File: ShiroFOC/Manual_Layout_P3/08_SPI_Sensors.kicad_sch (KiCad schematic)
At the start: 15 parts, among them U601 AS5047P-ATSM, U701 BMI323

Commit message: CAN layout
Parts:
- C601: symbol Manual:COMP_C601 -> ShiroFOCLib:COMP_C601
- C602: symbol Manual:COMP_C602 -> ShiroFOCLib:COMP_C602
- C701: symbol Manual:COMP_C701 -> ShiroFOCLib:COMP_C701
- C702: symbol Manual:COMP_C702 -> ShiroFOCLib:COMP_C702
- R308, R715: symbol Manual:COMP_R308 -> ShiroFOCLib:COMP_R308
- R309: symbol Manual:COMP_R309 -> ShiroFOCLib:COMP_R309
- R313: symbol Manual:COMP_R313 -> ShiroFOCLib:COMP_R313
- R314: symbol Manual:COMP_R314 -> ShiroFOCLib:COMP_R314
- R611: symbol Manual:COMP_R611 -> ShiroFOCLib:COMP_R611
- TP1010: symbol Manual:COMP_TP1010 -> ShiroFOCLib:COMP_TP1010
- TP1011: symbol Manual:COMP_TP1011 -> ShiroFOCLib:COMP_TP1011
- TP1012: symbol Manual:COMP_TP1012 -> ShiroFOCLib:COMP_TP1012
- U601: footprint Manual:AS5047P_TSSOP14 -> ShiroFOCLib:AS5047P_TSSOP14; symbol Manual:COMP_U601 -> ShiroFOCLib:COMP_U601
- U701: footprint Manual:BMI323_LGA14 -> ShiroFOCLib:BMI323_LGA14; symbol Manual:COMP_U701_I2C -> ShiroFOCLib:COMP_U701_I2C
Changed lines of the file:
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@@
 	)
 	(symbol
-		(lib_id "Manual:COMP_C702")
+		(lib_id "ShiroFOCLib:COMP_C702")
 		(at 195.58 168.91 0)
 		(unit 1)
@@
 	)
 	(symbol
-		(lib_id "Manual:COMP_TP1012")
+		(lib_id "ShiroFOCLib:COMP_TP1012")
 		(at 120.65 93.98 0)
 		(unit 1)
@@
 	)
 	(symbol
-		(lib_id "Manual:COMP_TP1011")
+		(lib_id "ShiroFOCLib:COMP_TP1011")
 		(at 109.22 104.14 0)
 		(unit 1)
@@
 	)
 	(symbol
-		(lib_id "Manual:PWR_3V3")
+		(lib_id "ShiroFOCLib:PWR_3V3")
 		(at 154.94 38.1 0)
 		(unit 1)
@@
 	)
 	(symbol
-		(lib_id "Manual:PWR_3V3")
+		(lib_id "ShiroFOCLib:PWR_3V3")
 		(at 180.34 180.34 0)
 		(unit 1)
@@
 	)
 	(symbol
-		(lib_id "Manual:PWR_3V3")
+		(lib_id "ShiroFOCLib:PWR_3V3")
 		(at 96.52 177.8 0)
 		(unit 1)
@@
 	)
 	(symbol
-		(lib_id "Manual:PWR_GND")
+		(lib_id "ShiroFOCLib:PWR_GND")
 		(at 180.34 137.16 0)
 		(unit 1)
@@
 	)
 	(symbol
-		(lib_id "Manual:COMP_U601")
+		(lib_id "ShiroFOCLib:COMP_U601")
 		(at 175.26 96.52 0)
 		(unit 1)
@@
 			)
 		)
-		(property "Footprint" "Manual:AS5047P_TSSOP14"
+		(property "Footprint" "ShiroFOCLib:AS5047P_TSSOP14"
 			(at 175.26 129.54 0)
 			(effects
@@
 	)
 	(symbol
-		(lib_id "Manual:COMP_R309")
+		(lib_id "ShiroFOCLib:COMP_R309")
 		(at 223.52 59.69 0)
 		(unit 1)
@@
 	)
 	(symbol
-		(lib_id "Manual:PWR_GND")
+		(lib_id "ShiroFOCLib:PWR_GND")
 		(at 170.18 246.38 0)
 		(unit 1)
@@
 	)
 	(symbol
-		(lib_id "Manual:COMP_R313")
+		(lib_id "ShiroFOCLib:COMP_R313")
 		(at 101.6 83.82 0)
 		(unit 1)
@@
 	)
 	(symbol
-		(lib_id "Manual:COMP_C601")
+		(lib_id "ShiroFOCLib:COMP_C601")
 		(at 154.94 48.26 0)
 		(unit 1)
@@
 	)
 	(symbol
-		(lib_id "Manual:PWR_3V3")
+		(lib_id "ShiroFOCLib:PWR_3V3")
 		(at 180.34 55.88 0)
 		(unit 1)
@@
 	)
 	(symbol
-		(lib_id "Manual:PWR_3V3")
+		(lib_id "ShiroFOCLib:PWR_3V3")
 		(at 170.18 55.88 0)
 		(unit 1)
@@
 	)
 	(symbol
-		(lib_id "Manual:COMP_C602")
+		(lib_id "ShiroFOCLib:COMP_C602")
 		(at 195.58 48.26 0)
 		(unit 1)
@@
 	)
 	(symbol
-		(lib_id "Manual:PWR_3V3")
+		(lib_id "ShiroFOCLib:PWR_3V3")
 		(at 223.52 187.96 0)
 		(unit 1)
@@
 	)
 	(symbol
-		(lib_id "Manual:PWR_GND")
+		(lib_id "ShiroFOCLib:PWR_GND")
 		(at 170.18 137.16 0)
 		(unit 1)
@@
 	)
 	(symbol
-		(lib_id "Manual:COMP_C701")
+		(lib_id "ShiroFOCLib:COMP_C701")
 		(at 154.94 168.91 0)
 		(unit 1)
@@
 	)
 	(symbol
-		(lib_id "Manual:COMP_R308")
+		(lib_id "ShiroFOCLib:COMP_R308")
 		(at 96.52 187.96 0)
 		(unit 1)
@@
 	)
 	(symbol
-		(lib_id "Manual:PWR_GND")
+		(lib_id "ShiroFOCLib:PWR_GND")
 		(at 148.59 226.06 0)
 		(unit 1)
@@
 	)
 	(symbol
-		(lib_id "Manual:PWR_GND")
+		(lib_id "ShiroFOCLib:PWR_GND")
 		(at 154.94 58.42 0)
 		(unit 1)
@@
 	)
 	(symbol
-		(lib_id "Manual:PWR_GND")
+		(lib_id "ShiroFOCLib:PWR_GND")
 		(at 195.58 179.07 0)
 		(unit 1)
@@
 	)
 	(symbol
-		(lib_id "Manual:COMP_R308")
+		(lib_id "ShiroFOCLib:COMP_R308")
 		(at 121.92 187.96 0)
 		(unit 1)
@@
 	)
 	(symbol
-		(lib_id "Manual:PWR_3V3")
+		(lib_id "ShiroFOCLib:PWR_3V3")
 		(at 195.58 38.1 0)
 		(unit 1)
@@
 	)
 	(symbol
-		(lib_id "Manual:COMP_R611")
+		(lib_id "ShiroFOCLib:COMP_R611")
 		(at 130.81 104.14 0)
 		(unit 1)
@@
 	)
 	(symbol
-		(lib_id "Manual:PWR_3V3")
+		(lib_id "ShiroFOCLib:PWR_3V3")
 		(at 121.92 177.8 0)
 		(unit 1)
@@
 	)
 	(symbol
-		(lib_id "Manual:PWR_GND")
+		(lib_id "ShiroFOCLib:PWR_GND")
 		(at 180.34 246.38 0)
 		(unit 1)
@@
 	)
 	(symbol
-		(lib_id "Manual:COMP_TP1010")
+		(lib_id "ShiroFOCLib:COMP_TP1010")
 		(at 120.65 83.82 0)
 		(unit 1)
@@
 	)
 	(symbol
-		(lib_id "Manual:PWR_GND")
+		(lib_id "ShiroFOCLib:PWR_GND")
 		(at 154.94 179.07 0)
 		(unit 1)
@@
 	)
 	(symbol
-		(lib_id "Manual:PWR_3V3")
+		(lib_id "ShiroFOCLib:PWR_3V3")
 		(at 223.52 49.53 0)
 		(unit 1)
@@
 	)
 	(symbol
-		(lib_id "Manual:PWR_3V3")
+		(lib_id "ShiroFOCLib:PWR_3V3")
 		(at 195.58 158.75 0)
 		(unit 1)
@@
 	)
 	(symbol
-		(lib_id "Manual:PWR_3V3")
+		(lib_id "ShiroFOCLib:PWR_3V3")
 		(at 170.18 180.34 0)
 		(unit 1)
@@
 	)
 	(symbol
-		(lib_id "Manual:COMP_U701_I2C")
+		(lib_id "ShiroFOCLib:COMP_U701_I2C")
 		(at 175.26 213.36 0)
 		(unit 1)
@@
 			)
 		)
-		(property "Footprint" "Manual:BMI323_LGA14"
+		(property "Footprint" "ShiroFOCLib:BMI323_LGA14"
 			(at 175.26 238.76 0)
 			(effects
@@
 	)
 	(symbol
-		(lib_id "Manual:PWR_GND")
+		(lib_id "ShiroFOCLib:PWR_GND")
 		(at 195.58 58.42 0)
 		(unit 1)
@@
 	)
 	(symbol
-		(lib_id "Manual:PWR_3V3")
+		(lib_id "ShiroFOCLib:PWR_3V3")
 		(at 154.94 158.75 0)
 		(unit 1)
@@
 	)
 	(symbol
-		(lib_id "Manual:COMP_R314")
+		(lib_id "ShiroFOCLib:COMP_R314")
 		(at 101.6 93.98 0)
 		(unit 1)

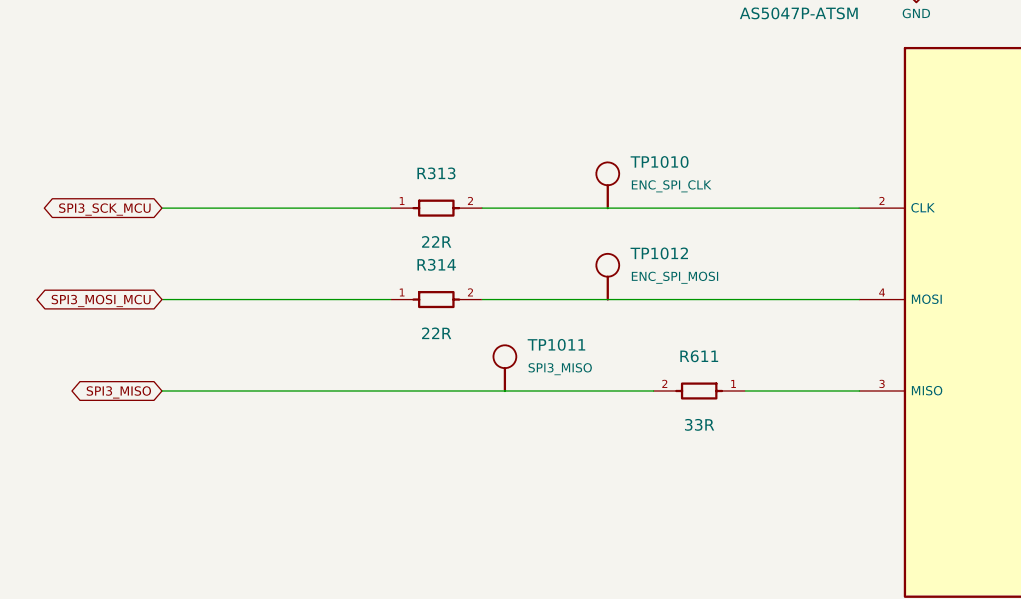
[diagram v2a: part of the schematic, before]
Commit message: most caps placed
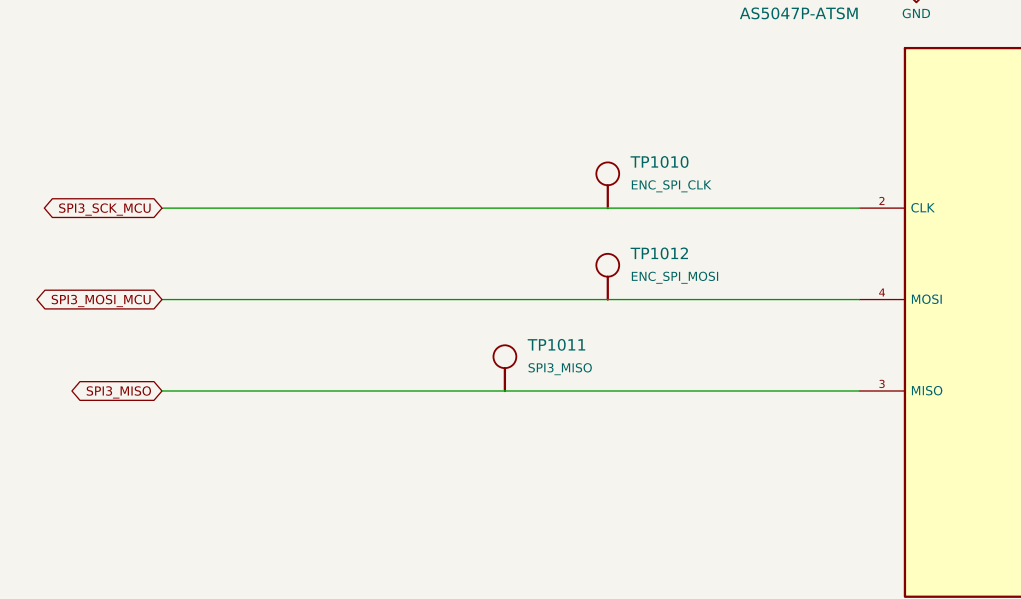
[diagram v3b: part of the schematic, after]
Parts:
- removed R313: 22R, Resistor_SMD:R_0402_1005Metric, symbol ShiroFOCLib:COMP_R313
- removed R314: 22R, Resistor_SMD:R_0402_1005Metric, symbol ShiroFOCLib:COMP_R314
- removed R611: 33R, Resistor_SMD:R_0402_1005Metric, symbol ShiroFOCLib:COMP_R611
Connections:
- net SPI3_MISO: now also U601.3 (MISO)
- net SPI3_MOSI_MCU: now also TP1012.1, U601.4 (MOSI)
- net SPI3_SCK_MCU: now also TP1010.1, U601.2 (CLK)
